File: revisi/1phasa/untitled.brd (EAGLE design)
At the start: 80 x 102 mm, 55 parts, among them J1 U.FL-R-SMT(01), J2 10118193-0001LF, K2 SRD-05VDC-SL-C, Q1 S9013, Q16 MMBT3904, Q17 MMBT3904, Q18 12MHz, U1 AMS1117, U19 CH340G, U2 PC817X2NIP0F, U3 ESP32-WROOM-32D

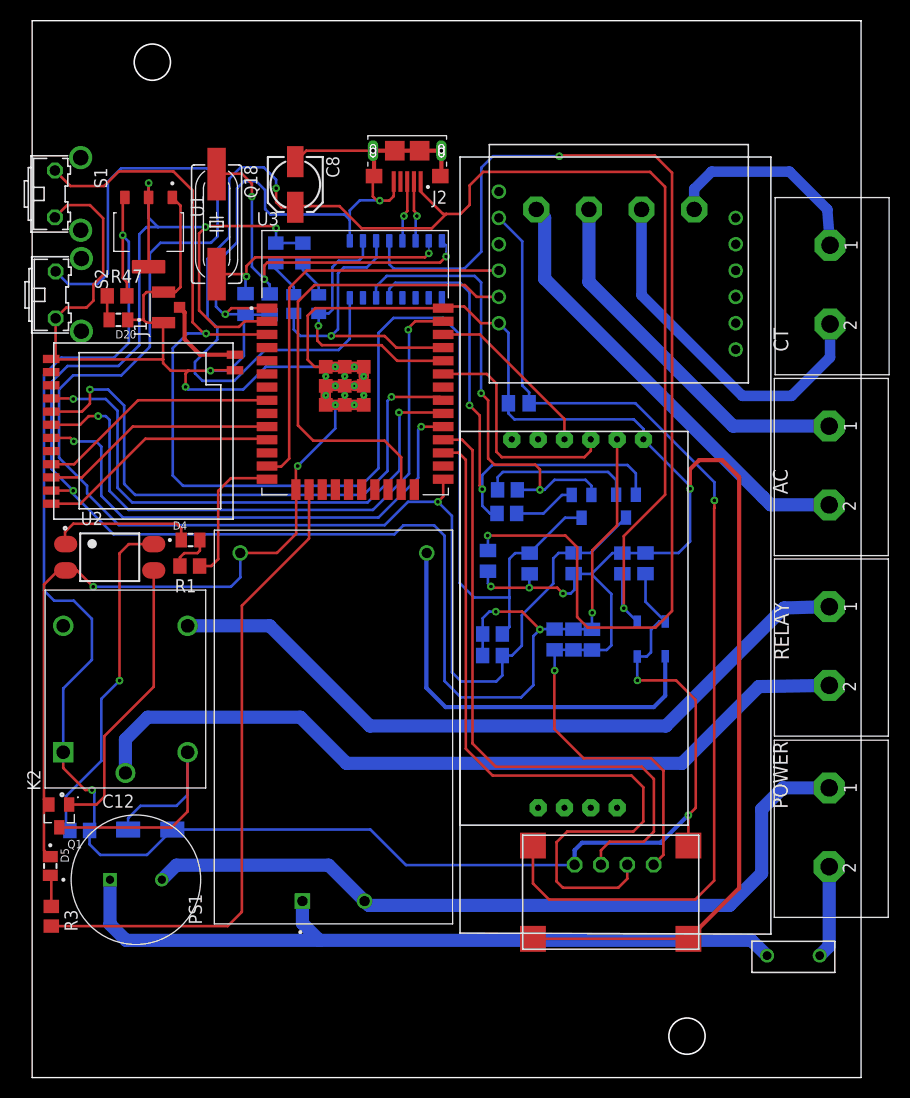
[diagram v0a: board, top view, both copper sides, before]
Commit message: revisi tanggal 07/01/2023
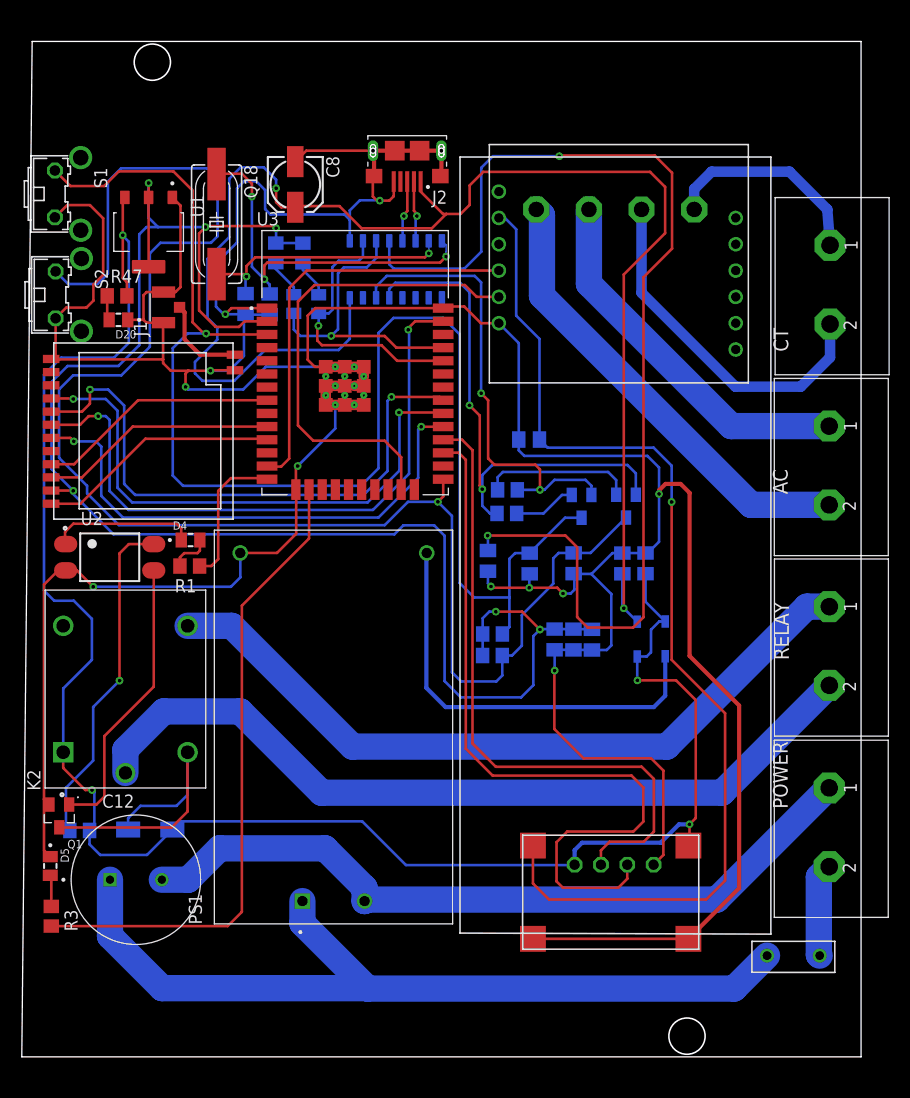
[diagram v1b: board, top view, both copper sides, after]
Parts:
- removed RTC1: (no value), rtc3231:RTC3231
- moved C13 3.64 mm to (48.0, 50.6)
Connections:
- net 3V3: no longer RTC1.VCC
- net GND: no longer RTC1.GND
- net SCL: no longer RTC1.SCL
- net SDA: no longer RTC1.SDA
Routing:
- net SDA: track 22.8 -> 0.00 mm
- net 3V3: track 182.7 -> 163.4 mm, vias 7 -> 6
- net SCL: track 17.0 -> 0.00 mm
- net N$1: track 73.4 -> 83.3 mm
- net GND: track 451.7 -> 444.6 mm
- net N$9: track 77.0 -> 79.3 mm
- net N$2: track 74.9 -> 73.0 mm
- net N$13: track 101.1 -> 102.9 mm
- net N$10: track 70.7 -> 72.4 mm
- net N$104: track 109.5 -> 108.2 mm
- net N$15: track 43.5 -> 44.6 mm
- net N$17: track 35.2 -> 34.4 mm
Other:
- board size 80 x 102 mm -> 81 x 98 mm
